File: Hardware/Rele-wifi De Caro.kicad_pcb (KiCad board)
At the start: 2 copper layers, 11 parts, among them J1 Screw_Terminal_01x03, J2 Screw_Terminal_01x03, J3 Screw_Terminal_01x03, J4 Screw_Terminal_01x03, J5 Screw_Terminal_01x02, Q2 PC817-B, Q4 PC817-B, Q5 PC817-B, Q7 PC817-B, U2 ESP32-CAM, U3 LM7805_TO220

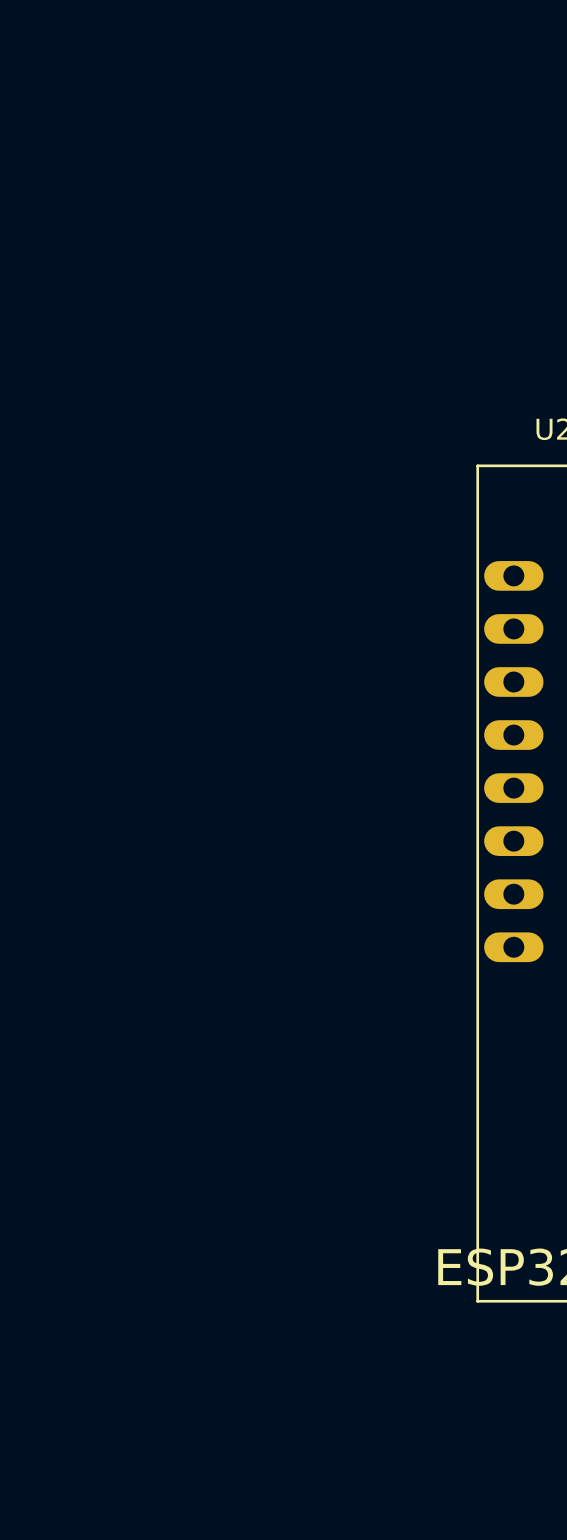
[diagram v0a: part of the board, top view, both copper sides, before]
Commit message: Avance de esquematico
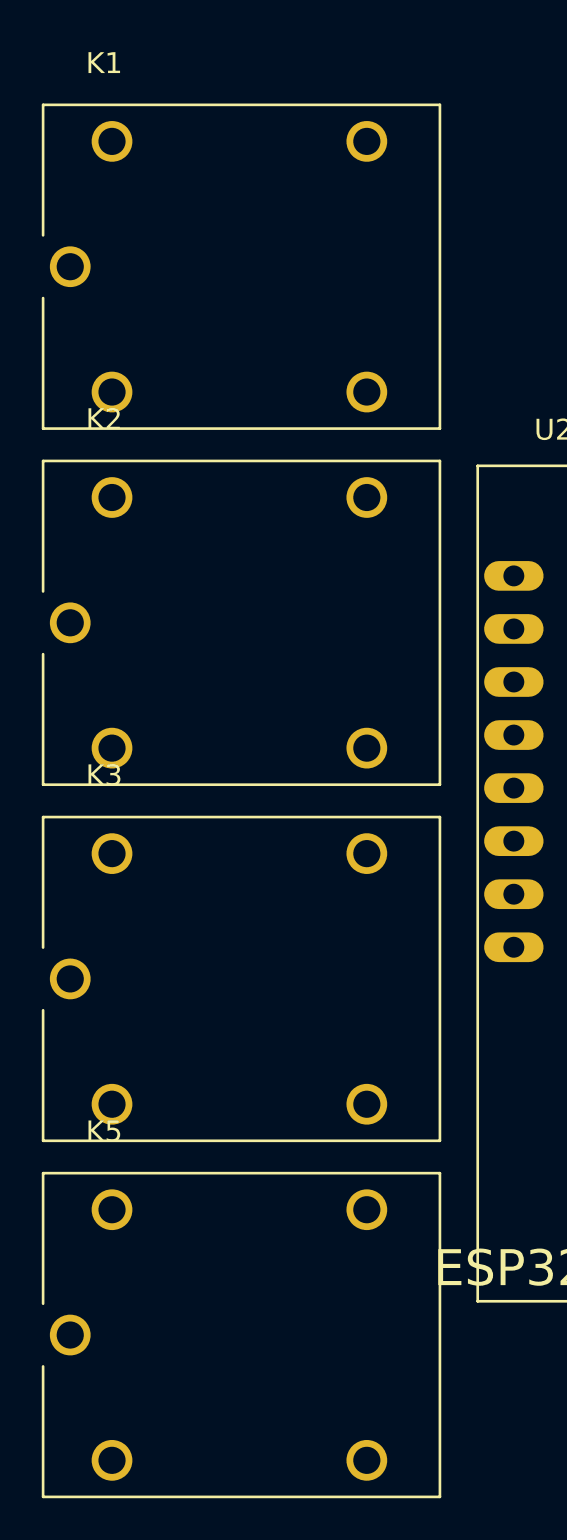
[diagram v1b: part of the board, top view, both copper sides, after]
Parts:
- added K1: Relay_SPDT, Relay:RELAY_PR13-5V-450-1C, F.Cu at (107.0, 60.3)
- added K2: Relay_SPDT, Relay:RELAY_PR13-5V-450-1C, F.Cu at (107.0, 77.4)
- added K3: Relay_SPDT, Relay:RELAY_PR13-5V-450-1C, F.Cu at (107.0, 94.4)
- added K5: Relay_SPDT, Relay:RELAY_PR13-5V-450-1C, F.Cu at (107.0, 111.5)
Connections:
- U2 pad P$1: Net-(U1-OUT) -> Net-(U2-5V)
- U3 pad 1: unconnected-(U3-VI-Pad1) -> Net-(SW1A-B)
- U3 pad 2: unconnected-(U3-GND-Pad2) -> GND
- U3 pad 3: unconnected-(U3-VO-Pad3) -> Net-(U2-5V)
